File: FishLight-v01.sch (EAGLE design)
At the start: 71 parts, among them U1 SPARK_CORECORE, U10 AD5248MSOP-10, U11 INA219SOT23-8, U12 INA219SOT23-8, U13 INA219SOT23-8, U14 INA219SOT23-8, U15 INA219SOT23-8, U16 UA7812D2PAK-3, U17 L7805D2PAK-2, U18 RK7002BSOT23-3, U19 RK7002BSOT23-3, U2 RTCBREAKOUT, U20 RELAY-SOLIDSTATEPTH, U21 RELAY-SOLIDSTATEPTH, U3 CAT4101TO-263, U4 CAT4101TO-263, U5 CAT4101TO-263, U6 CAT4101TO-263, U7 CAT4101TO-263, U8 AD5248MSOP-10, U9 AD5248MSOP-10

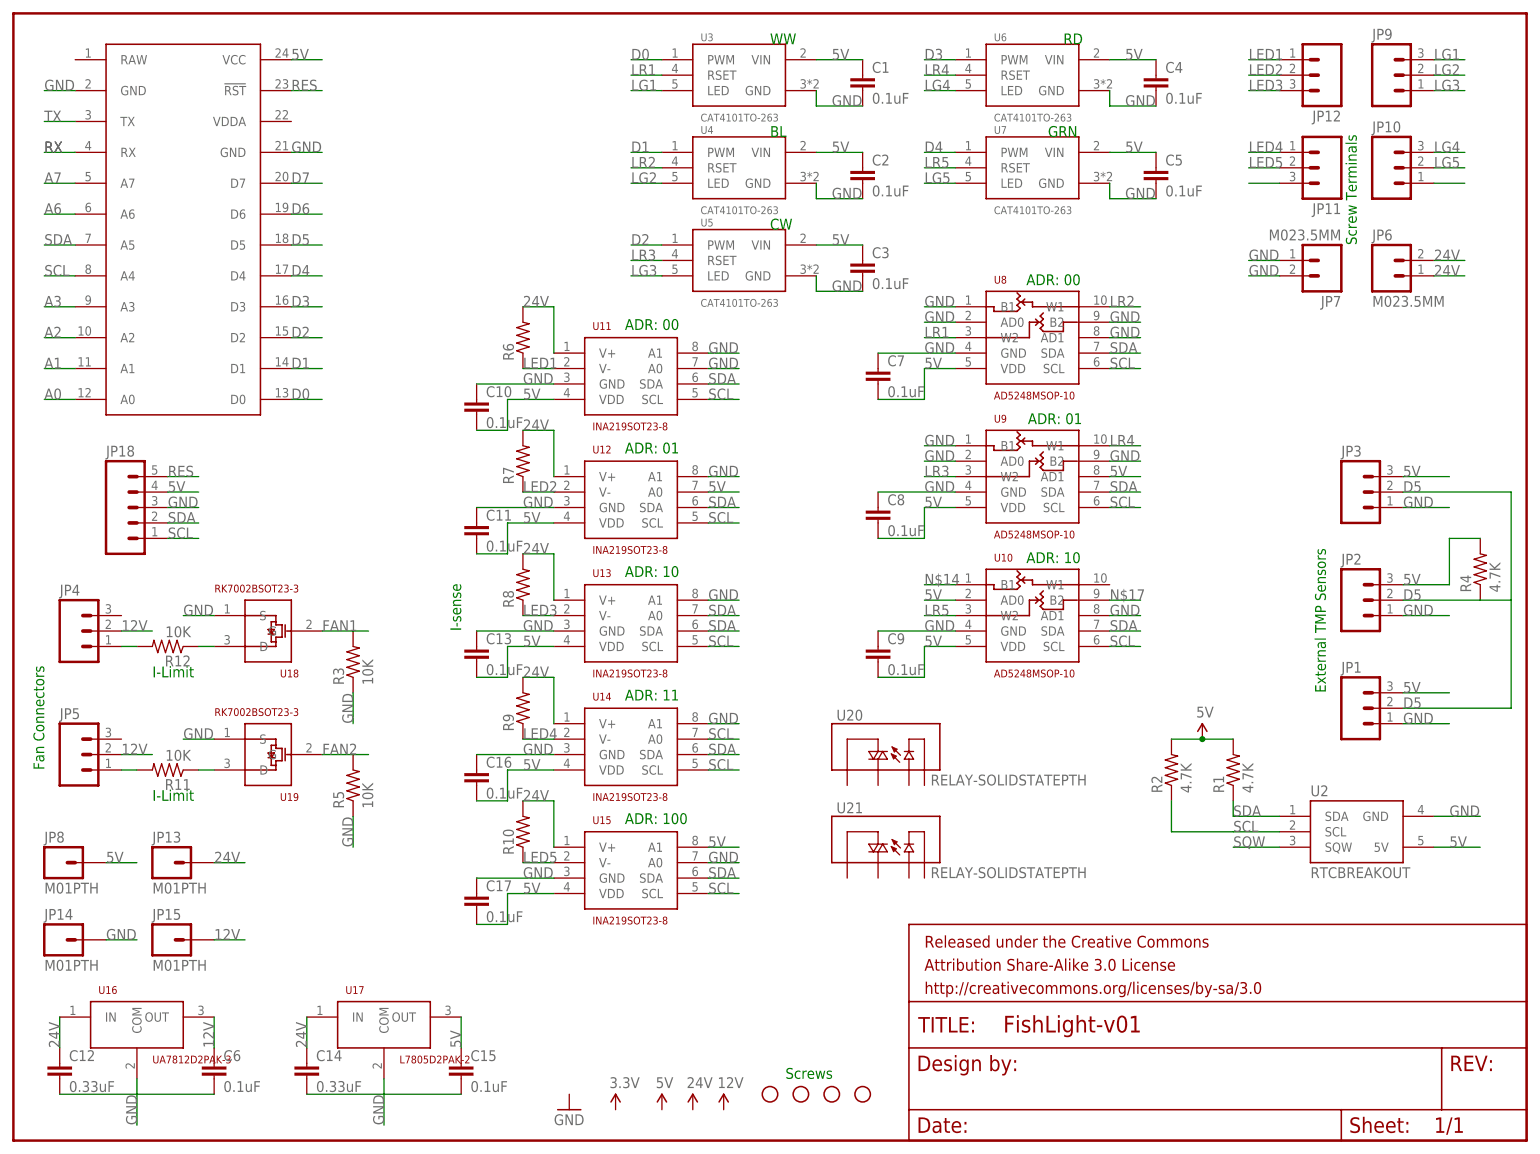
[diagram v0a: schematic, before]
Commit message: FishLight_PCB: Added LED strings 4 - 8
Added LED strings 4 - 8 and removed the 'green' string.  This will allow
me to control 2 tanks or one really big tank in the future.  Added all
of the accompanying parts and moved a lot of stuff around to make it all
fit on the schematic.  Still need to lay them out on the board tho.
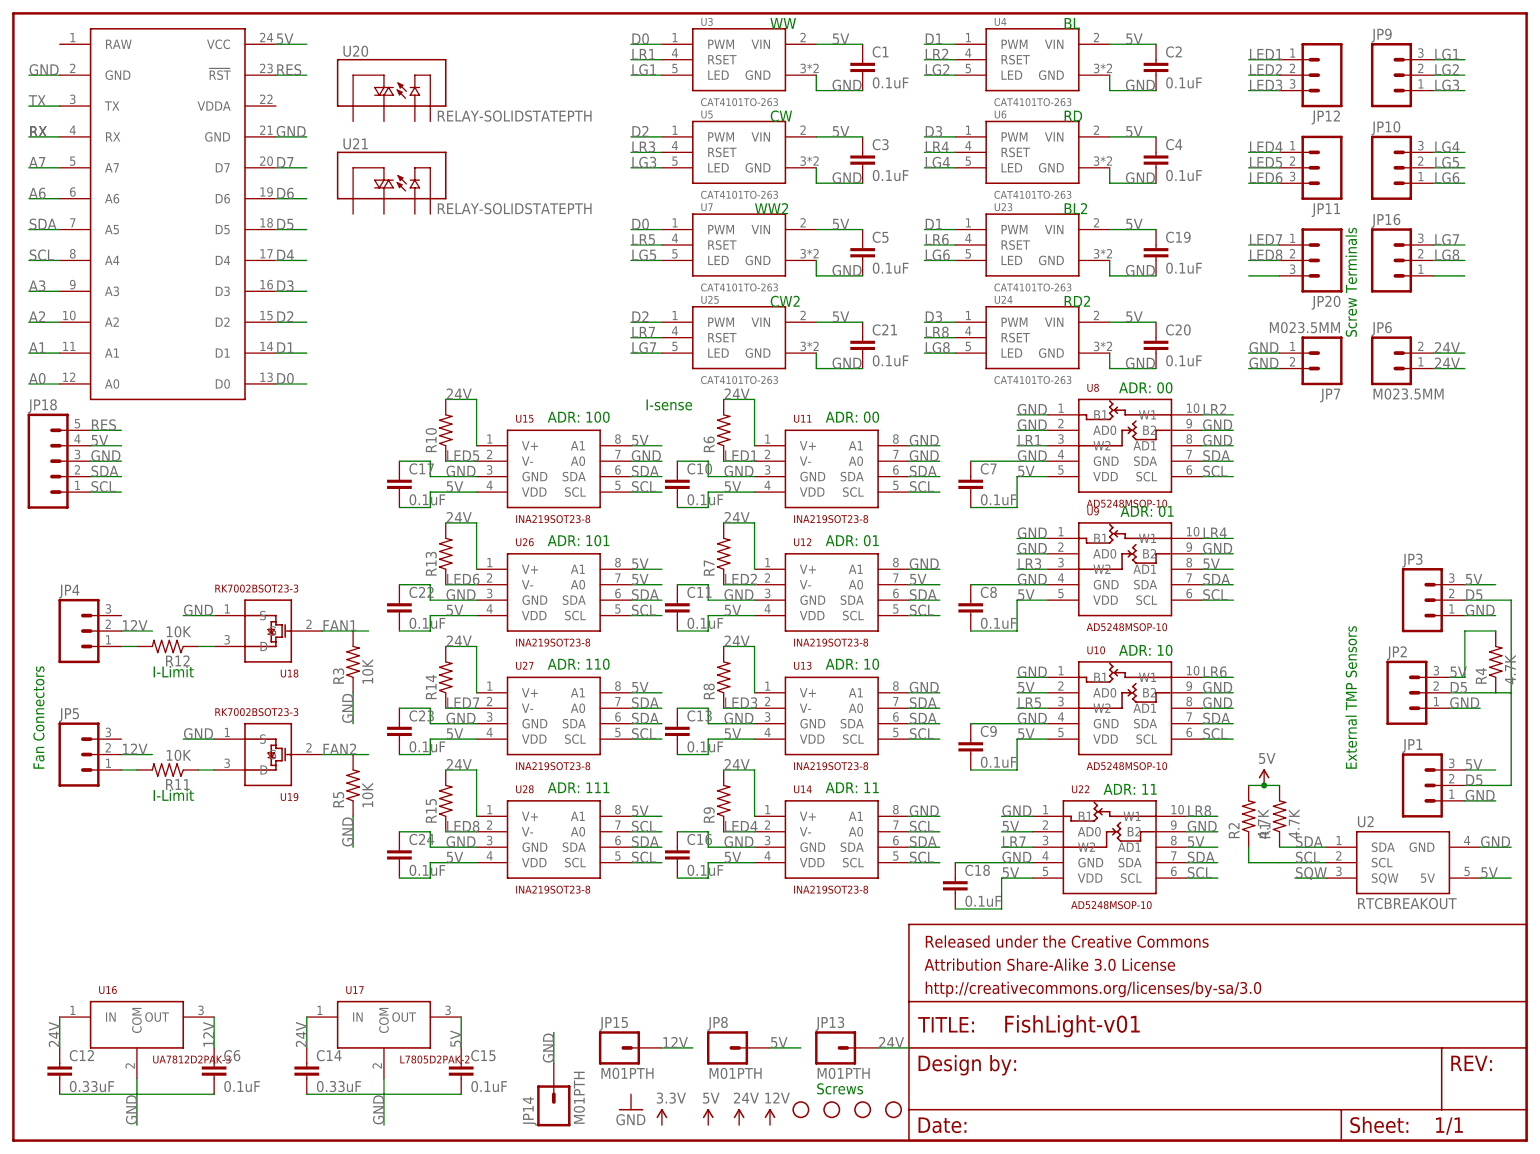
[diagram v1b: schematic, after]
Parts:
- added C18, C19, C20, C21, C22, C23, C24: 0.1uF, SparkFun-Capacitors:0.1UF-25V(+80/-20%)(0603)
- added JP16, JP20: (no value), Mikes-Stuff:M03SCREW
- added R13, R14, R15: (no value), SparkFun-Resistors:RESISTOR2010
- added U22: AD5248MSOP-10, Mikes-Stuff:AD5248MSOP-10
- added U23, U24, U25: CAT4101TO-263, Mikes-Stuff:CAT4101TO-263
- added U26, U27, U28: INA219SOT23-8, Mikes-Stuff:INA219SOT23-8
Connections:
- removed net N$14: U10.B1
- removed net N$17: U10.B2
- removed net N$3: JP11.3
- removed net N$6: JP10.1
- new net LED6: JP11.3, R13.1, U26.V-
- new net LED7: JP20.1, R14.1, U27.V-
- new net LED8: JP20.2, R15.1, U28.V-
- new net LG6: JP10.1, U23.LED
- new net LG7: JP16.3, U25.LED
- new net LG8: JP16.2, U24.LED
- new net LR6: U10.W1, U23.RSET
- new net LR7: U22.W2, U25.RSET
- new net LR8: U22.W1, U24.RSET
- new net N$22: JP20.3
- new net N$27: JP16.1
- net 24V: now also R13.2, R14.2, R15.2, U26.V+, U27.V+, U28.V+
- net 5V: now also C18.2, C19.1, C20.1, C21.1, C22.2, C23.2, C24.2, U12.A0, U22.AD0, U22.AD1, U22.VDD, U23.VIN, U24.VIN, U25.VIN, U26.A0, U26.A1, U26.VDD, U27.A1, U27.VDD, U28.A1, U28.VDD
- net D0: now also U7.PWM
- net D1: now also U23.PWM
- net D2: now also U25.PWM
- net D3: now also U24.PWM
- net D4: no longer U7.PWM
- net GND: now also C18.1, C19.2, C20.2, C21.2, C22.1, C23.1, C24.1, U10.B1, U10.B2, U11.A0, U11.A1, U12.A1, U13.A1, U22.B1, U22.B2, U22.GND, U23.GND, U24.GND, U25.GND, U26.GND, U27.GND, U28.GND
- net SCL: now also U11.SCL, U12.SCL, U13.SCL, U22.SCL, U26.SCL, U27.SCL, U28.A0, U28.SCL
- net SDA: now also U11.SDA, U12.SDA, U13.A0, U13.SDA, U22.SDA, U26.SDA, U27.A0, U27.SDA, U28.SDA
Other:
- note added: "ADR: 101"
- note added: "ADR: 110"
- note added: "ADR: 111"
- note added: "BL2"
- note added: "CW2"
- note added: "RD2"
- note added: "WW2"
- note removed: "GRN"
- moved on the sheet: C1, C10, C11, C13, C16, C17, C2, C3, C4, C5, C7, C8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
